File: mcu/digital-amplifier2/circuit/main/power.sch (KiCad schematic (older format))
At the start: 35 parts, among them J5 Barrel_Jack_Switch, U3 TPS54360DDA, U4 AMS1117-3.3, U5 LT3045xMSE-1

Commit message: save
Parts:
- U5: symbol misc:LT3045xMSE-1 -> digital-amplifier2-rescue:LT3045xMSE-1-misc
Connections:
- net +3.3VA: now also U5.13 (GND)
- net GND: no longer U5.13 (GND)
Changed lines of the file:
@@
 $EndComp
 $Comp
-L misc:LT3045xMSE-1 U?
+L digital-amplifier2-rescue:LT3045xMSE-1-misc U?
 U 1 1 5FBE4493
 P 7550 1975
@@
 AR Path="/5FBB5CE4/5FBE4493" Ref="U?"  Part="1"
 AR Path="/5F16021E/5FBE4493" Ref="U5"  Part="1"
+AR Path="/5FBE4493" Ref="U5"  Part="1"
 F 0 "U5" H 7550 2442 50  0000 C CNN
 F 1 "LT3045xMSE-1" H 7550 2351 50  0000 C CNN

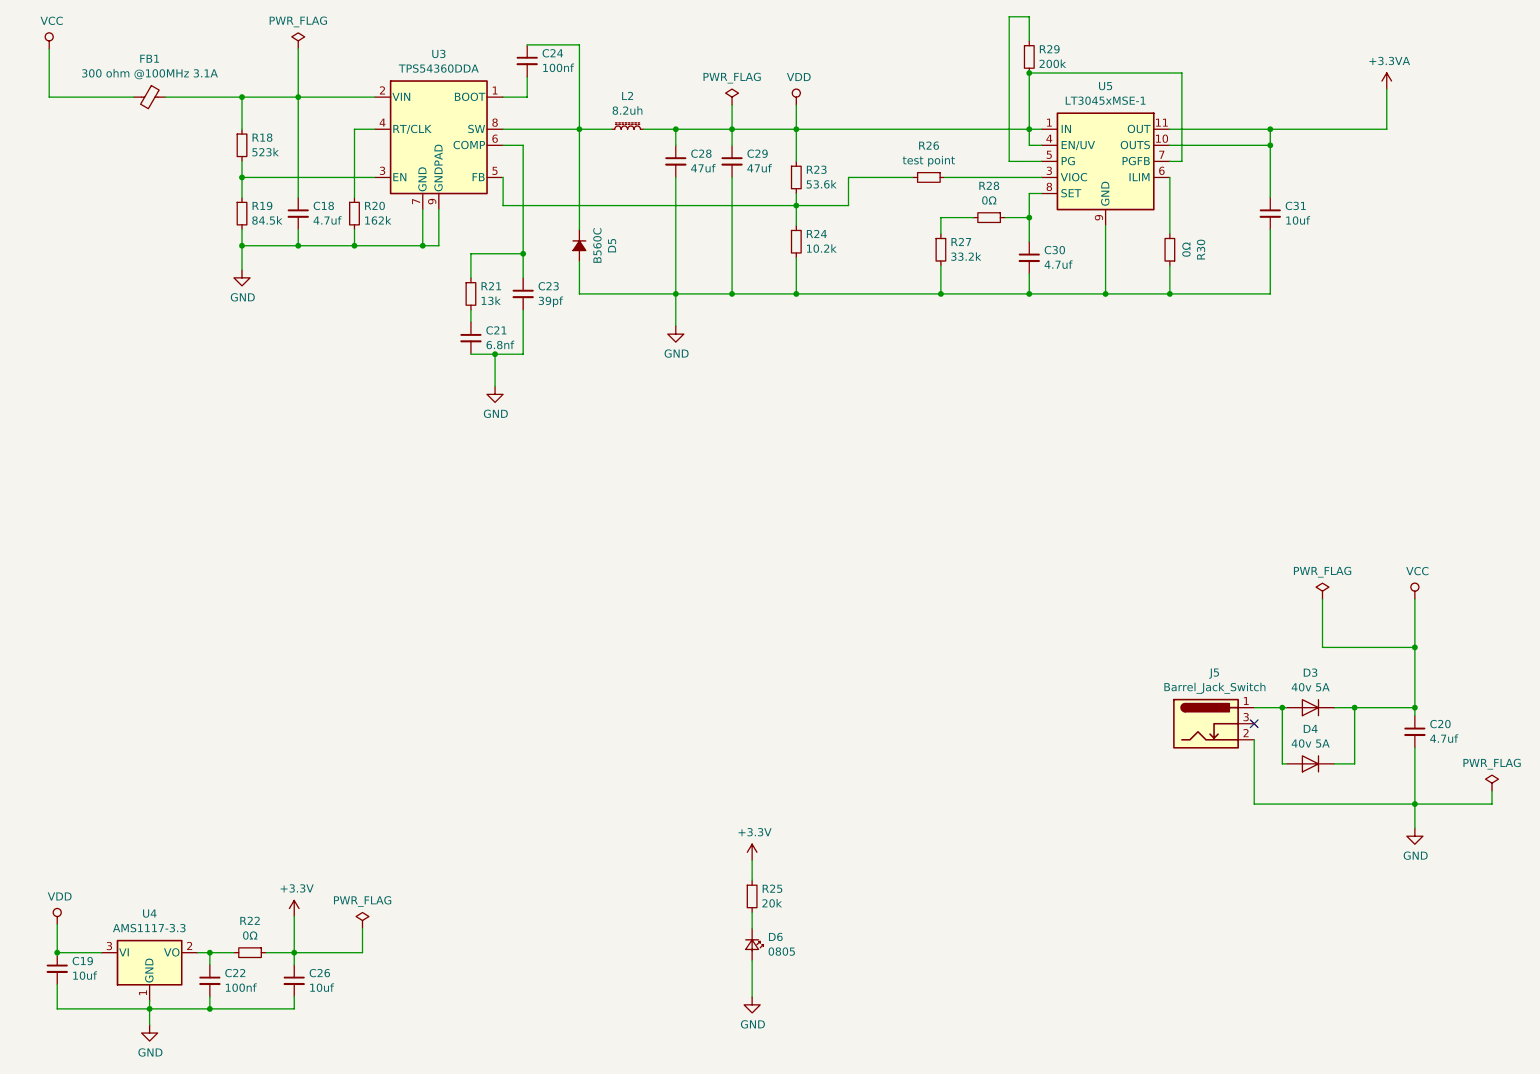
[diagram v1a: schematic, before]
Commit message: headphone
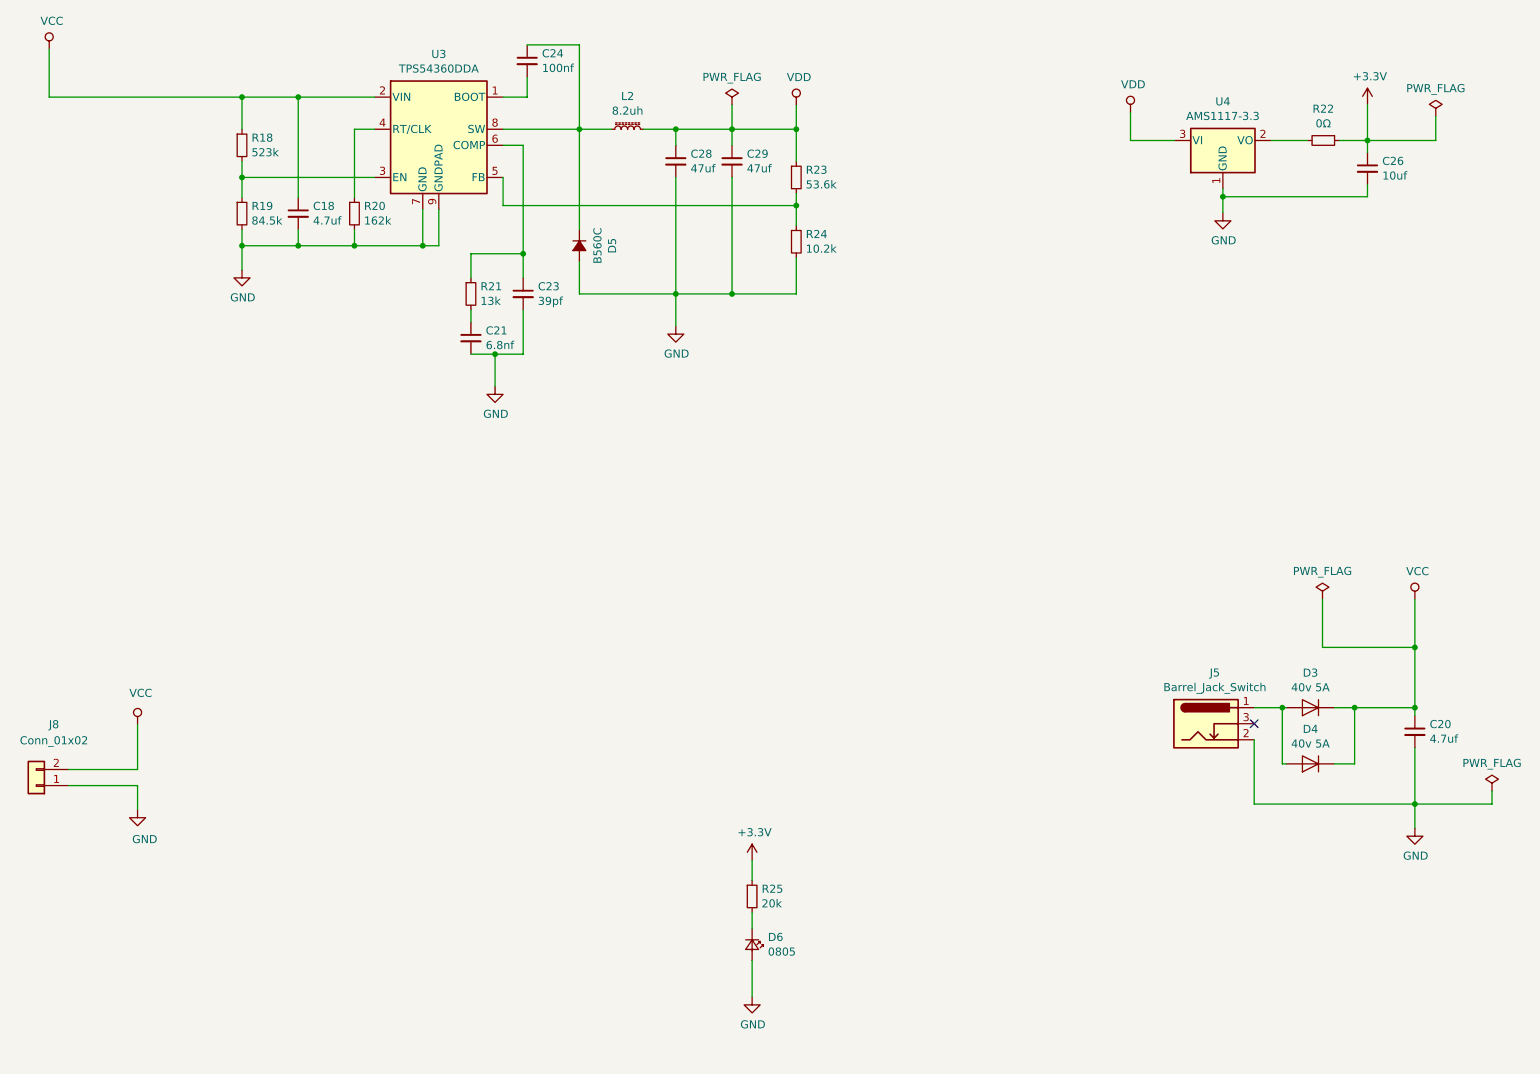
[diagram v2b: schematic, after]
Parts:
- removed C19, C31: 10uf, Capacitor_SMD:C_0805_2012Metric, symbol Device:C_Small
- removed C22: 100nf, Capacitor_SMD:C_0805_2012Metric, symbol Device:C_Small
- removed C30: 4.7uf, Capacitor_SMD:C_0805_2012Metric, symbol Device:C_Small
- removed FB1: 300 ohm @100MHz 3.1A, Inductor_SMD:L_1210_3225Metric, symbol Device:Ferrite_Bead_Small
- removed R26: test point, Resistor_SMD:R_0805_2012Metric, symbol Device:R_Small
- removed R27: 33.2k, Resistor_SMD:R_0805_2012Metric, symbol Device:R_Small
- removed R28, R30: 0Ω, Resistor_SMD:R_0805_2012Metric, symbol Device:R_Small
- removed R29: 200k, Resistor_SMD:R_0805_2012Metric, symbol Device:R_Small
- removed U5: LT3045xMSE-1, Package_SO:MSOP-12-1EP_3x4mm_P0.65mm_EP1.65x2.85mm, symbol digital-amplifier2-rescue:LT3045xMSE-1-misc
- added J8: Conn_01x02, Connector_JST:JST_VH_S2P-VH_1x02_P3.96mm_Horizontal, symbol Connector_Generic:Conn_01x02
- J5: footprint Connector_BarrelJack:BarrelJack_Horizontal -> connector:DC-044A_5.5-2.1
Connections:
- net GND: now also J8.1 (Pin_1)
- net VCC: now also C18.1, R18.1, U3.2 (VIN), J8.2 (Pin_2)
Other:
- moved on the sheet: C26, R22, U4
